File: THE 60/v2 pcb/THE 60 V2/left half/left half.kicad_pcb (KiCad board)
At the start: 2 copper layers, 141.7 x 107.7 mm, 70 parts, among them J2 Conn_01x02_Socket, SW3 Switch, SW4 Switch, U1 Nice_Nano_V2, U4 TRRS

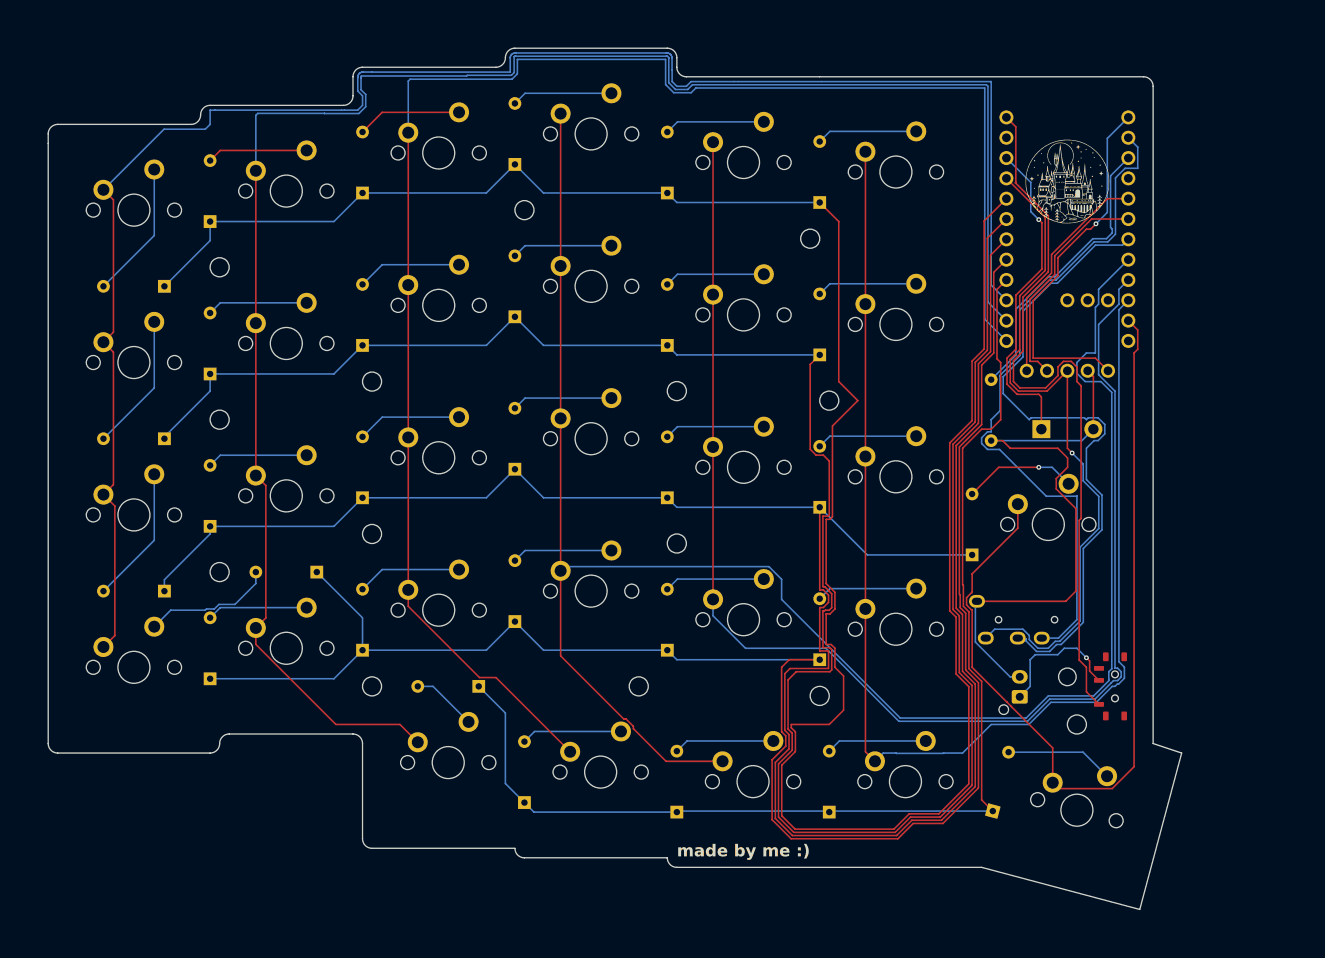
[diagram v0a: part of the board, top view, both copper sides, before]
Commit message: z
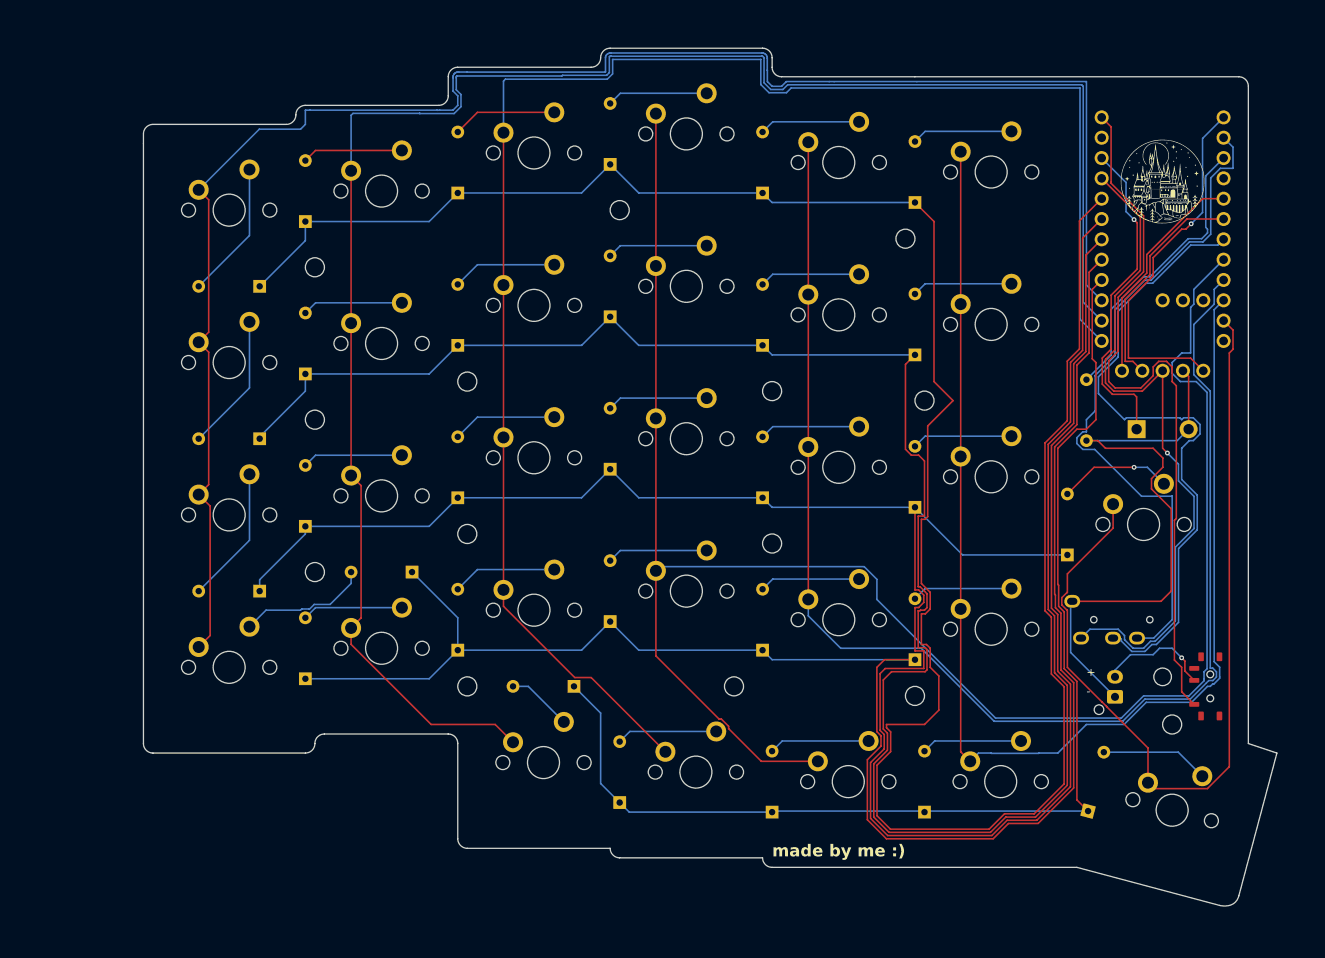
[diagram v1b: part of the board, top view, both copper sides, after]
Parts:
- moved D30 11.9 mm to (197.3, 116.6)
- moved D31 11.9 mm to (199.9, 148.6)
- moved D32 11.9 mm to (178.2, 72.5)
- moved D33 11.9 mm to (178.2, 91.6)
- moved D34 11.9 mm to (178.2, 110.6)
- moved D35 11.9 mm to (178.2, 129.7)
- moved D36 11.9 mm to (159.2, 71.3)
- moved D37 11.9 mm to (159.2, 90.4)
- moved D38 11.9 mm to (159.2, 109.4)
- moved D39 11.9 mm to (159.2, 128.5)
- moved D40 11.9 mm to (160.4, 148.7)
- moved D41 11.9 mm to (140.1, 67.8)
- moved D42 11.9 mm to (140.1, 86.8)
- moved D43 11.9 mm to (140.1, 105.9)
- moved D44 11.9 mm to (140.1, 124.9)
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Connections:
- J2 pad 1: +. -> gnd.
- J2 pad 2: gnd. -> +.
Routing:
- net +.: track 16.8 -> 14.3 mm
- net gnd.: track 75.1 -> 76.9 mm
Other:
- board size 141.7 x 107.7 mm -> 141.7 x 107.2 mm
- board text added: "+"
- board text added: "-"

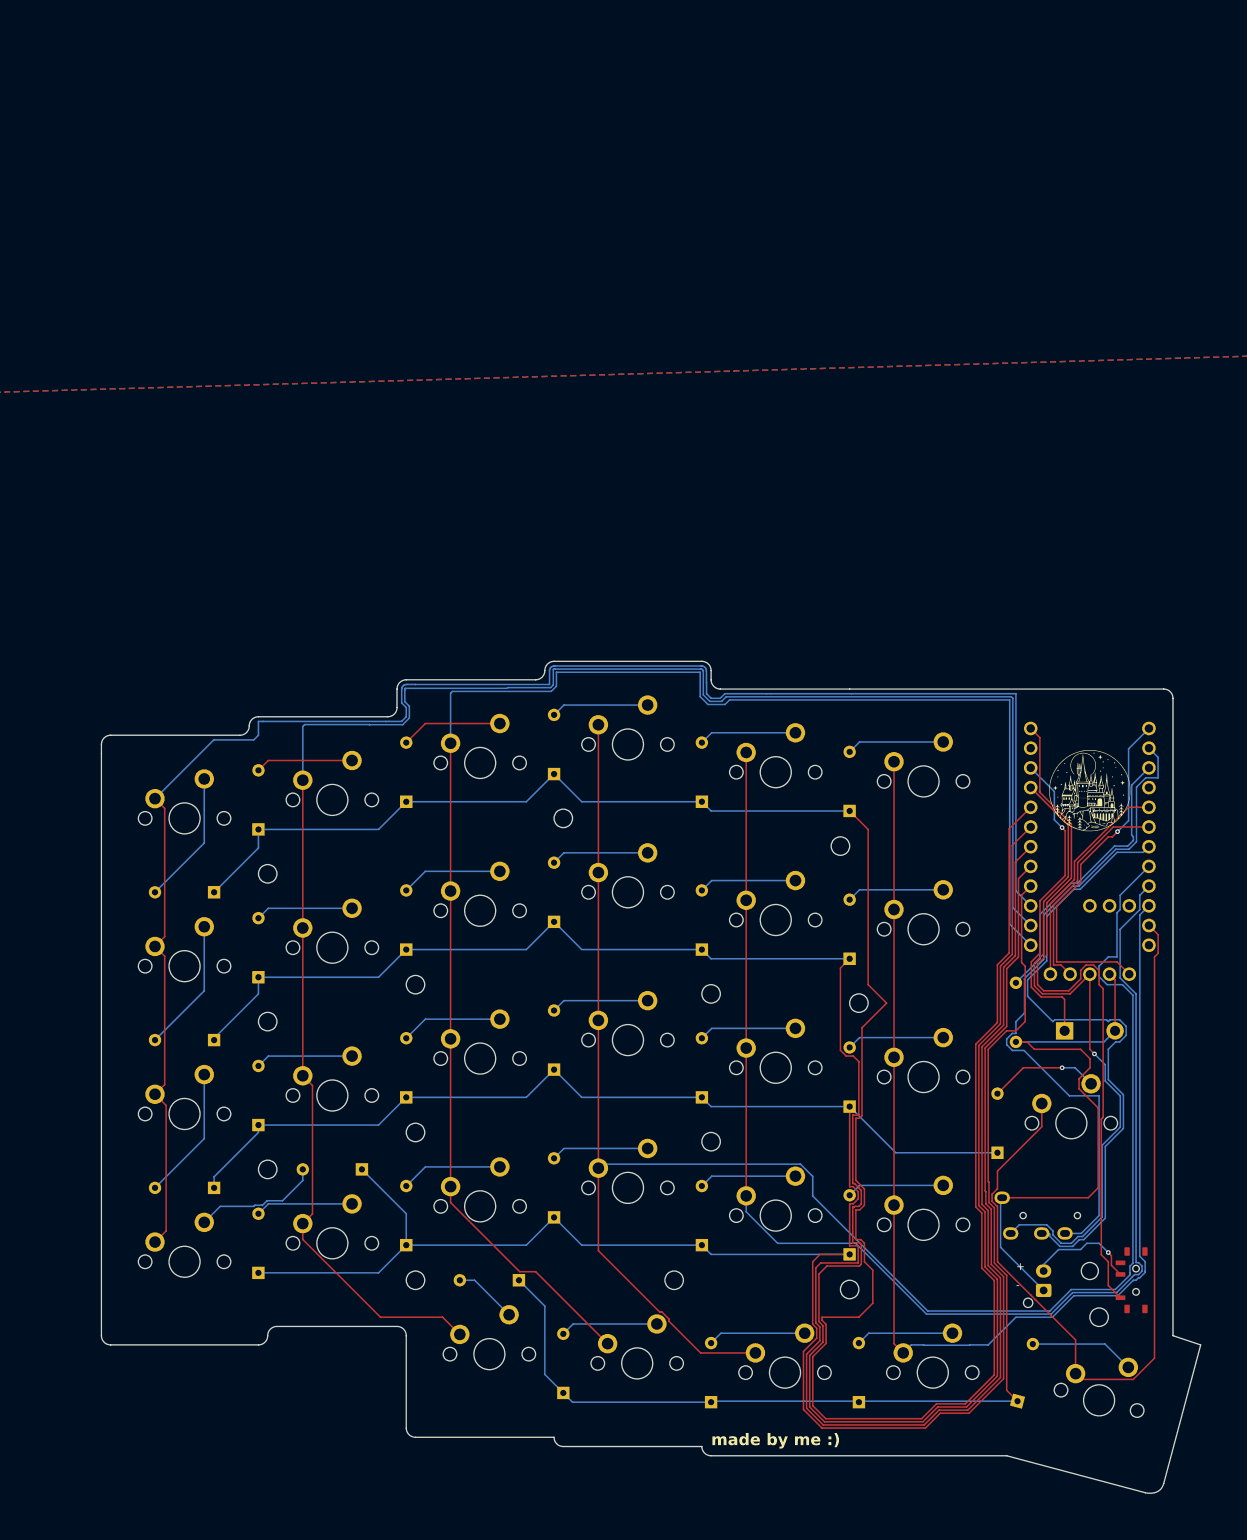
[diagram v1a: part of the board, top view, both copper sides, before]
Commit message: UPLOADED THE layout json
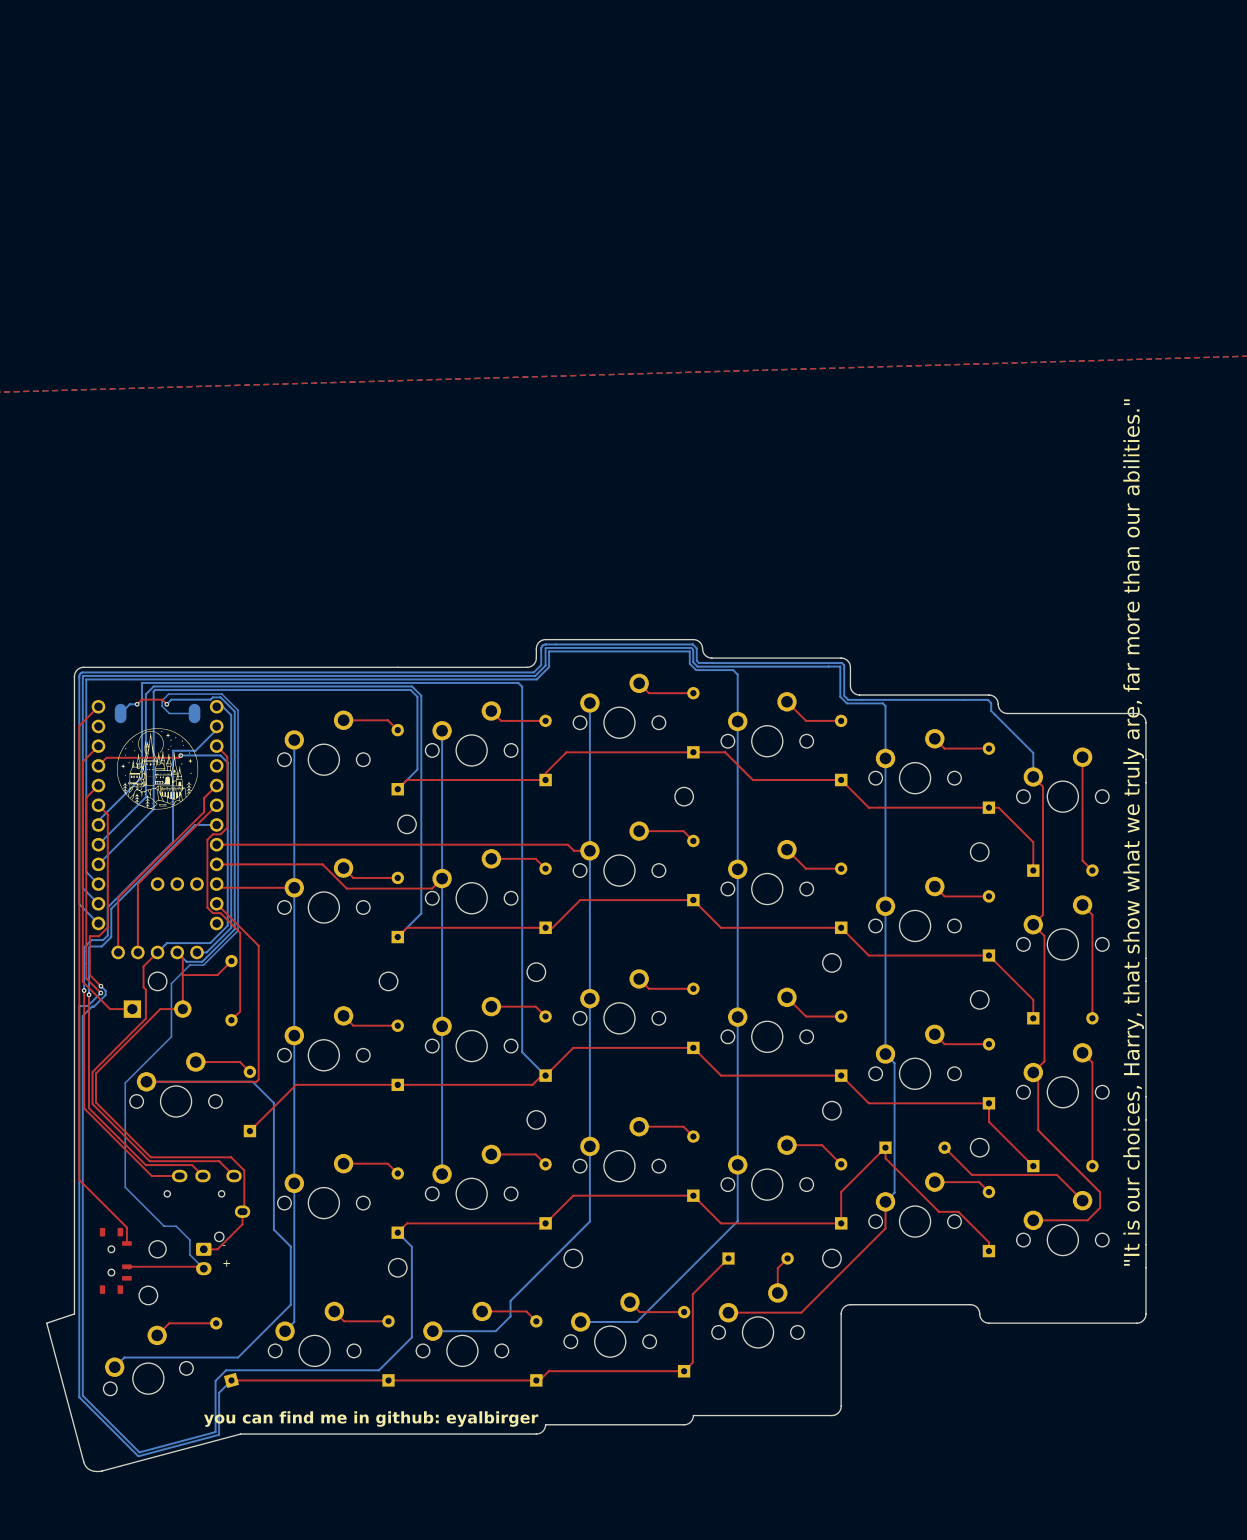
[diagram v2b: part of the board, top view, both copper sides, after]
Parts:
- removed D30, D31, D32, D33, D34, D35, D36, D37, D38, D39, D40, D41, D42, D43, D44, D45, D46, D47, D48, D49, D50, D51, D52, D53, D54, D55, D56, D57, D58, D60: Diode, ScottoKeebs_Components:Diode_DO-35
- removed Display2: nice!view, nice view:nice_view
- removed the G*** at (180.6, 102.0)
- removed H12: MountingHole, MountingHole:MountingHole_2.2mm_M2
- removed J2: Conn_01x02_Socket, Connector_JST:JST_XH_B2B-XH-AM_1x02_P2.50mm_Vertical
- removed R2: Resistor, Resistor_THT:R_Axial_DIN0207_L6.3mm_D2.5mm_P7.62mm_Horizontal
- removed S30, S31, S32, S33, S34, S35, S36, S37, S38, S39, S40, S41, S42, S43, S44, S45, S46, S47, S48, S49, S50, S51, S52, S53, S54, S55, S56, S57, S58, S60: Keyswitch, ScottoKeebs_MX:MX_PCB_1.00u
- removed SW3: Switch, ScottoKeebs_Components:Switch_MSK12C02
- removed SW4: Switch, ScottoKeebs_Components:Button_MJTP1243
- removed U1: Nice_Nano_V2, ScottoKeebs_MCU:Nice_Nano_V2_Flipped
- removed U4: TRRS, ScottoKeebs_Components:TRRS_PJ-320A
- added D1: Diode, ScottoKeebs_Components:Diode_DO-35, B.Cu at (120.0, 69.7)
- added D10: Diode, ScottoKeebs_Components:Diode_DO-35, B.Cu at (177.2, 87.6)
- added D11: Diode, ScottoKeebs_Components:Diode_DO-35, B.Cu at (196.2, 91.1)
- added D12: Diode, ScottoKeebs_Components:Diode_DO-35, B.Cu at (201.9, 99.2)
- added D13: Diode, ScottoKeebs_Components:Diode_DO-35, B.Cu at (120.0, 107.8)
- added D14: Diode, ScottoKeebs_Components:Diode_DO-35, B.Cu at (139.1, 106.6)
- added D15: Diode, ScottoKeebs_Components:Diode_DO-35, B.Cu at (158.1, 103.1)
- added D16: Diode, ScottoKeebs_Components:Diode_DO-35, B.Cu at (177.2, 106.6)
- added D17: Diode, ScottoKeebs_Components:Diode_DO-35, B.Cu at (196.2, 110.2)
- added D18: Diode, ScottoKeebs_Components:Diode_DO-35, B.Cu at (201.9, 118.3)
- added D19: Diode, ScottoKeebs_Components:Diode_DO-35, B.Cu at (120.0, 126.9)
- added D2: Diode, ScottoKeebs_Components:Diode_DO-35, B.Cu at (139.1, 68.5)
- added D20: Diode, ScottoKeebs_Components:Diode_DO-35, B.Cu at (139.1, 125.7)
- added D21: Diode, ScottoKeebs_Components:Diode_DO-35, B.Cu at (158.1, 122.1)
- added D22: Diode, ScottoKeebs_Components:Diode_DO-35, B.Cu at (177.2, 125.7)
- added D23: Diode, ScottoKeebs_Components:Diode_DO-35, B.Cu at (196.2, 129.2)
- added D24: Diode, ScottoKeebs_Components:Diode_DO-35, B.Cu at (182.9, 115.9)
- added D25: Diode, ScottoKeebs_Components:Diode_DO-35, B.Cu at (101.0, 113.8)
- added D26: Diode, ScottoKeebs_Components:Diode_DO-35, B.Cu at (162.6, 130.2)
- added D27: Diode, ScottoKeebs_Components:Diode_DO-35, B.Cu at (156.9, 144.7)
- added D28: Diode, ScottoKeebs_Components:Diode_DO-35, B.Cu at (137.9, 145.9)
- added D29: Diode, ScottoKeebs_Components:Diode_DO-35, B.Cu at (98.6, 145.9)
- added D3: Diode, ScottoKeebs_Components:Diode_DO-35, B.Cu at (158.1, 65.0)
- added D4: Diode, ScottoKeebs_Components:Diode_DO-35, B.Cu at (177.2, 68.5)
- added D5: Diode, ScottoKeebs_Components:Diode_DO-35, B.Cu at (196.2, 72.1)
- added D59: Diode, ScottoKeebs_Components:Diode_DO-35, B.Cu at (118.8, 145.9)
- added D6: Diode, ScottoKeebs_Components:Diode_DO-35, B.Cu at (201.9, 80.2)
- added D61: LED, custom:pad - oval2.5x1.5, B.Cu at (93.8, 60.0)
- added D62: LED, custom:pad - oval2.5x1.5, B.Cu at (84.3, 60.0)
- added D7: Diode, ScottoKeebs_Components:Diode_DO-35, B.Cu at (120.0, 88.8)
- added D8: Diode, ScottoKeebs_Components:Diode_DO-35, B.Cu at (139.1, 87.6)
- added D9: Diode, ScottoKeebs_Components:Diode_DO-35, B.Cu at (158.1, 84.0)
- added Display1: nice!view, nice view:nice_view, F.Cu at (89.0, 74.2)
- added G***: LOGO, logoo:hedwig leftttt, F.Cu at (116.4, 99.2)
- added G***: LOGO, logoo:the deathly hallows symbol, F.Cu at (200.4, 134.4)
- added H6: MountingHole, MountingHole:MountingHole_2.2mm_M2, F.Cu at (89.0, 129.0)
- added J1: Conn_01x02_Socket, Connector_JST:JST_XH_B2B-XH-AM_1x02_P2.50mm_Vertical, B.Cu at (95.0, 129.0)
- added R1: Resistor, Resistor_THT:R_Axial_DIN0207_L6.3mm_D2.5mm_P7.62mm_Horizontal, F.Cu at (98.6, 99.5)
- added S1: Keyswitch, ScottoKeebs_MX:MX_PCB_1.00u, F.Cu at (110.5, 65.9)
- added S10: Keyswitch, ScottoKeebs_MX:MX_PCB_1.00u, F.Cu at (167.6, 82.6)
- added S11: Keyswitch, ScottoKeebs_MX:MX_PCB_1.00u, F.Cu at (186.7, 87.3)
- added S12: Keyswitch, ScottoKeebs_MX:MX_PCB_1.00u, F.Cu at (205.7, 89.7)
- added S13: Keyswitch, ScottoKeebs_MX:MX_PCB_1.00u, F.Cu at (110.5, 104.0)
- added S14: Keyswitch, ScottoKeebs_MX:MX_PCB_1.00u, F.Cu at (129.5, 102.8)
- added S15: Keyswitch, ScottoKeebs_MX:MX_PCB_1.00u, F.Cu at (148.6, 99.2)
- added S16: Keyswitch, ScottoKeebs_MX:MX_PCB_1.00u, F.Cu at (167.6, 101.6)
- added S17: Keyswitch, ScottoKeebs_MX:MX_PCB_1.00u, F.Cu at (186.7, 106.4)
- added S18: Keyswitch, ScottoKeebs_MX:MX_PCB_1.00u, F.Cu at (205.7, 108.8)
- added S19: Keyswitch, ScottoKeebs_MX:MX_PCB_1.00u, F.Cu at (110.5, 123.1)
- added S2: Keyswitch, ScottoKeebs_MX:MX_PCB_1.00u, F.Cu at (129.5, 64.7)
- added S20: Keyswitch, ScottoKeebs_MX:MX_PCB_1.00u, F.Cu at (129.5, 121.9)
- added S21: Keyswitch, ScottoKeebs_MX:MX_PCB_1.00u, F.Cu at (148.6, 118.3)
- added S22: Keyswitch, ScottoKeebs_MX:MX_PCB_1.00u, F.Cu at (167.6, 120.7)
- added S23: Keyswitch, ScottoKeebs_MX:MX_PCB_1.00u, F.Cu at (186.7, 125.4)
- added S24: Keyswitch, ScottoKeebs_MX:MX_PCB_1.00u, F.Cu at (205.7, 127.8)
- added S25: Keyswitch, ScottoKeebs_MX:MX_PCB_1.00u, F.Cu at (91.4, 110.0)
- added S26: Keyswitch, ScottoKeebs_MX:MX_PCB_1.00u, F.Cu at (166.4, 139.7)
- added S27: Keyswitch, ScottoKeebs_MX:MX_PCB_1.00u, F.Cu at (147.4, 140.9)
- added S28: Keyswitch, ScottoKeebs_MX:MX_PCB_1.00u, F.Cu at (128.3, 142.1)
- added S29: Keyswitch, ScottoKeebs_MX:MX_PCB_1.00u, F.Cu at (87.9, 145.7)
- added S3: Keyswitch, ScottoKeebs_MX:MX_PCB_1.00u, F.Cu at (148.6, 61.1)
- added S4: Keyswitch, ScottoKeebs_MX:MX_PCB_1.00u, F.Cu at (167.6, 63.5)
- added S5: Keyswitch, ScottoKeebs_MX:MX_PCB_1.00u, F.Cu at (186.7, 68.3)
- added S59: Keyswitch, ScottoKeebs_MX:MX_PCB_1.00u, F.Cu at (109.3, 142.1)
- added S6: Keyswitch, ScottoKeebs_MX:MX_PCB_1.00u, F.Cu at (205.7, 70.7)
- added S7: Keyswitch, ScottoKeebs_MX:MX_PCB_1.00u, F.Cu at (110.5, 85.0)
- added S8: Keyswitch, ScottoKeebs_MX:MX_PCB_1.00u, F.Cu at (129.5, 83.8)
- added S9: Keyswitch, ScottoKeebs_MX:MX_PCB_1.00u, F.Cu at (148.6, 80.2)
- added SW1: Switch, ScottoKeebs_Components:Switch_MSK12C02, F.Cu at (83.1, 130.5)
- added SW2: Switch, ScottoKeebs_Components:Button_MJTP1243, F.Cu at (85.8, 98.1)
- added U2: Nice_Nano_V2, ScottoKeebs_MCU:Nice_Nano_V2_Flipped, F.Cu at (89.0, 73.0)
- added U3: TRRS, ScottoKeebs_Components:TRRS_PJ-320A, F.Cu at (88.7, 121.9)
- moved G*** 120.2 mm to (89.0, 67.1)
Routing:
- net row 0.: track 284.5 -> 0.00 mm
- net row 1.: track 262.2 -> 0.00 mm
- net row 2.: track 261.0 -> 0.00 mm
- net column 5: track 0.00 -> 242.5 mm
- net row 3: track 0.00 -> 242.5 mm, vias 0 -> 1
- net column 4: track 0.00 -> 235.8 mm
- net row 2: track 0.00 -> 234.3 mm
- net column 2.: track 232.7 -> 0.00 mm
- net column 4.: track 225.4 -> 0.00 mm
- net row 3.: track 217.3 -> 0.00 mm
- net column 5.: track 215.6 -> 0.00 mm
- net column 3: track 0.00 -> 211.9 mm
- net column 3.: track 204.2 -> 0.00 mm
- net row 4: track 0.00 -> 187.0 mm, vias 0 -> 1
- net row 1: track 0.00 -> 182.3 mm
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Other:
- outline, holes or cut-outs redrawn
- board text added: "you can find me in github: eyalbirger"
- board text added: "{dblquote}It is our choices, Harry, that show what we truly are, far more than our abilities.{dblquote}"
- board text added: "{dblquote}help will always be given at hogwarts to those who deserve it{dblquote}"
- board text removed: "Ring1"
- board text removed: "made by me :)"
